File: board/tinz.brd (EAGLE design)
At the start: 101.3 x 80 mm, 110 parts, among them U2 ATSAM3S4AA-AU

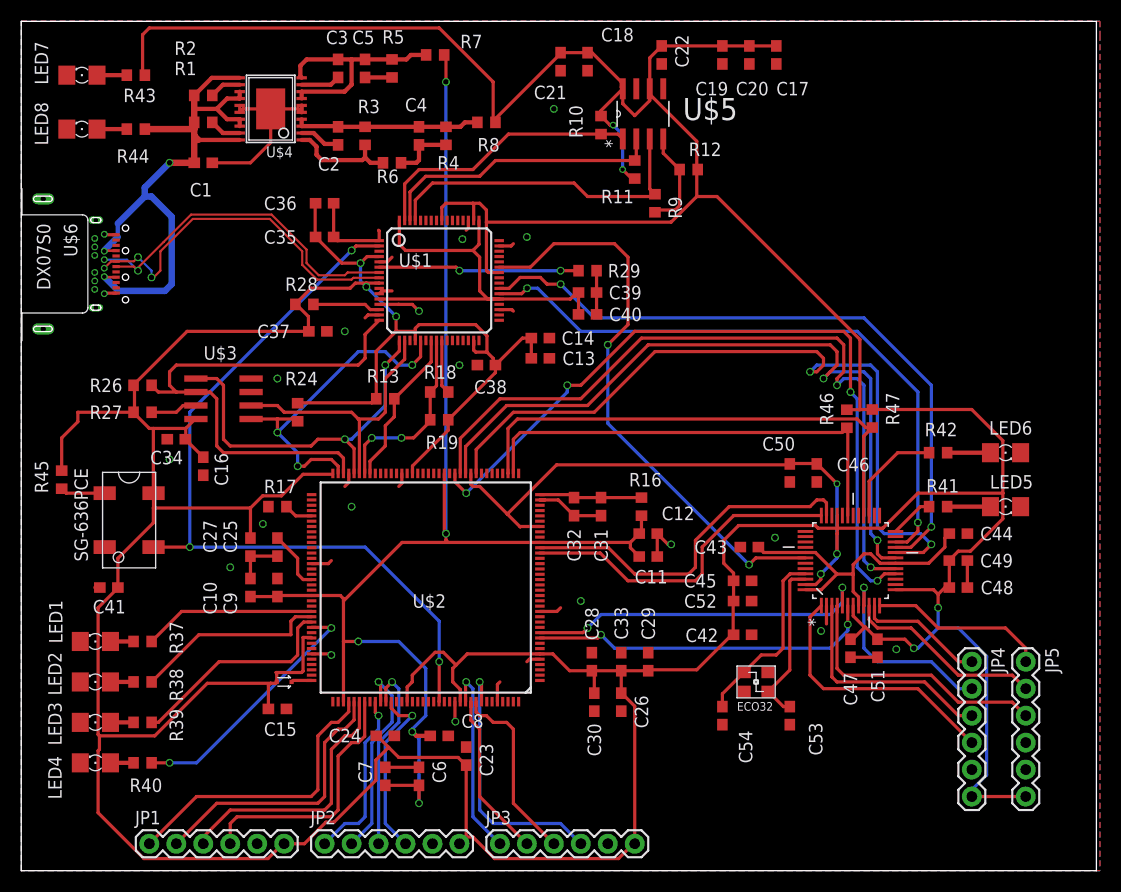
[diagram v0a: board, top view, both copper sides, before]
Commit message: Some minor changes.
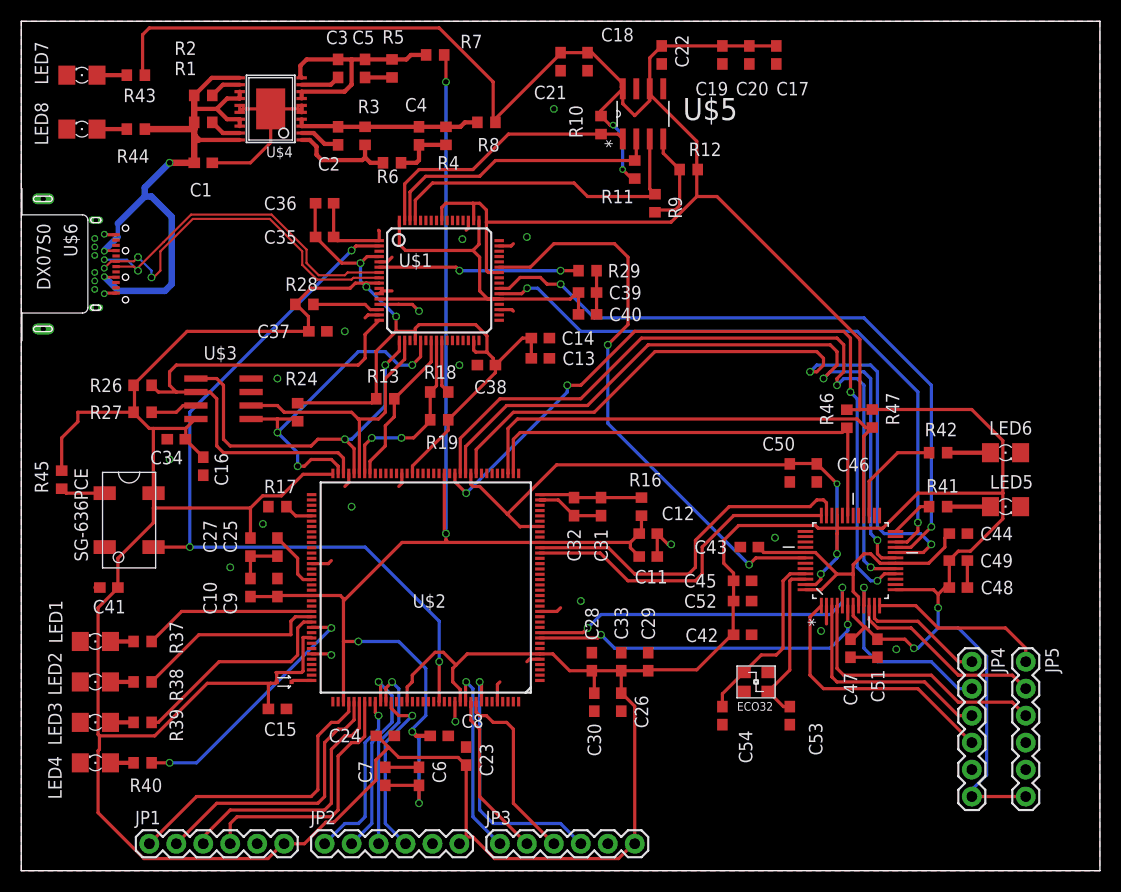
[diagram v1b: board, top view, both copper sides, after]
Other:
- board size 101.3 x 80 mm -> 101.6 x 80 mm
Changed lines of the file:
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@@
 <board>
 <plain>
-<wire x1="0" y1="0" x2="101.27" y2="0" width="0" layer="20"/>
-<wire x1="101.27" y1="0" x2="101.27" y2="80" width="0" layer="20"/>
-<wire x1="101.27" y1="80" x2="0" y2="80" width="0" layer="20"/>
-<wire x1="0" y1="80" x2="0" y2="0" width="0" layer="20"/>
+<wire x1="0" y1="0" x2="101.6" y2="0" width="0" layer="20"/>
+<wire x1="101.6" y1="0" x2="101.6" y2="80.01" width="0" layer="20"/>
+<wire x1="101.6" y1="80.01" x2="0" y2="80.01" width="0" layer="20"/>
+<wire x1="0" y1="80.01" x2="0" y2="0" width="0" layer="20"/>
 </plain>
 <attributes>
